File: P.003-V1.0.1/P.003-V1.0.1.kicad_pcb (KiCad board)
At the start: 2 copper layers, 19 parts, among them Q1 BS250, SW1 ON/OFF, SW2 Mode, SW3 Roll, U1 ATtiny85-20P, U2 74HC595

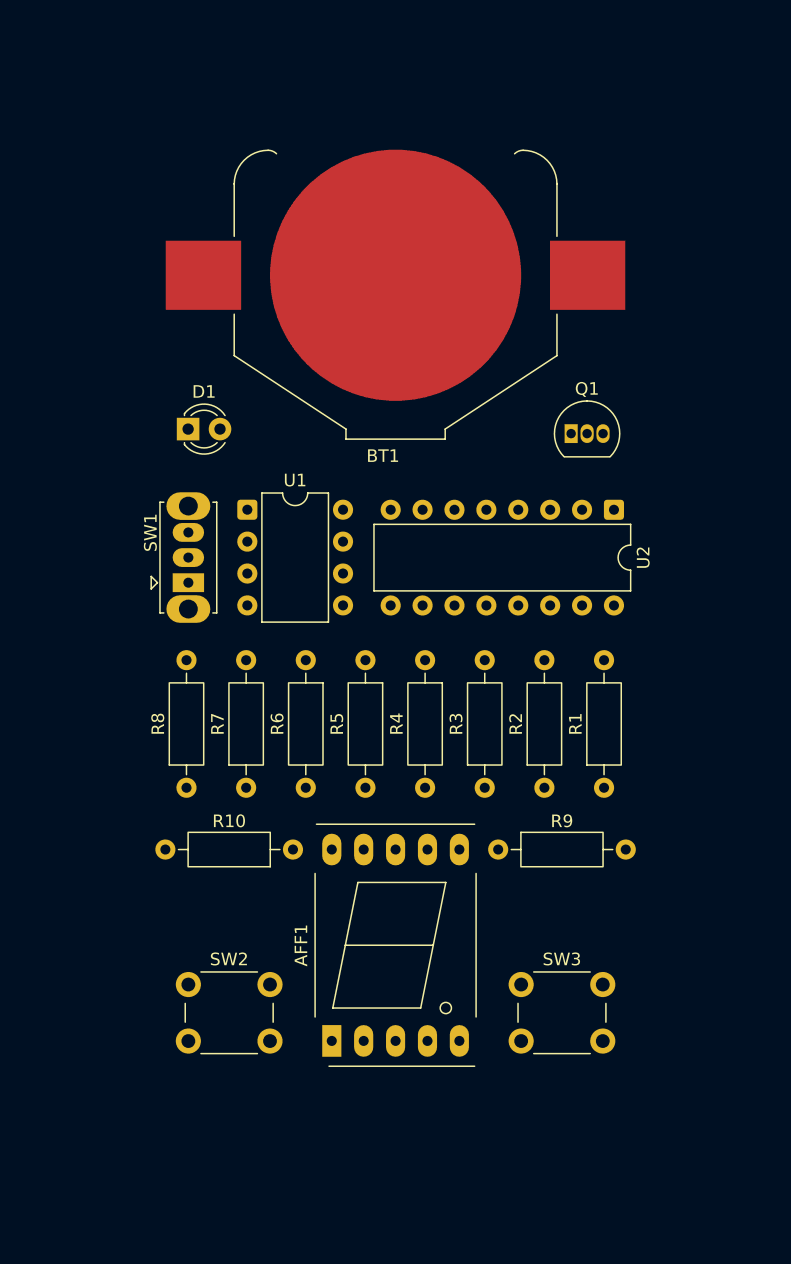
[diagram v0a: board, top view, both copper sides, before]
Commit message: add
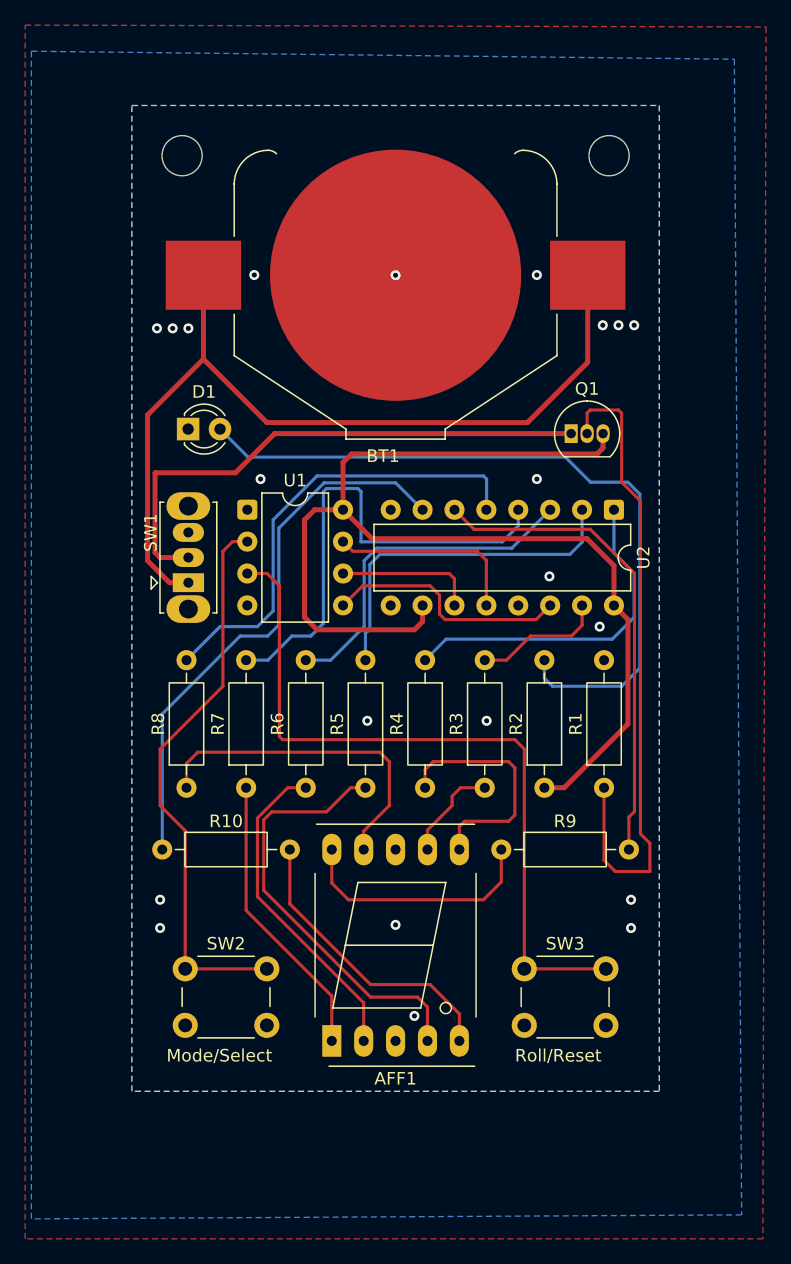
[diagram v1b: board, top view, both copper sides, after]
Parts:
- added ?: MountingHole_3.2mm_M3, MountingHole:MountingHole_3.2mm_M3, F.Cu at (112.0, 52.0)
- added ?: MountingHole_3.2mm_M3, MountingHole:MountingHole_3.2mm_M3, F.Cu at (146.0, 52.0)
- moved SW2 1.27 mm to (112.2, 116.7)
- moved SW3 1.27 mm to (139.2, 116.7)
- moved R10 0.25 mm to (120.6, 107.2)
- moved R9 0.25 mm to (137.4, 107.2)
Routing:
- net /Attiny85/VIN+: track 0.00 -> 93.8 mm
- net Net-(BT1-+): track 0.00 -> 70.2 mm
- net Net-(D1-A): track 0.00 -> 59.3 mm
- net Net-(U1-XTAL2/PB4): track 0.00 -> 58.9 mm
- net Net-(Q1-G): track 0.00 -> 51.8 mm
- net Net-(U1-XTAL1/PB3): track 0.00 -> 44.9 mm
- net /Display 7 Segment/Q7: track 0.00 -> 44.6 mm
- net Net-(Q1-D): track 0.00 -> 43.6 mm
- net /Display 7 Segment/Q4: track 0.00 -> 39.4 mm
- net /Display 7 Segment/Q6: track 0.00 -> 38.6 mm
- net /Display 7 Segment/Q5: track 0.00 -> 36.8 mm
- net Net-(AFF1-c): track 0.00 -> 34.4 mm
- net /Display 7 Segment/Q2: track 0.00 -> 28.0 mm
- net /Display 7 Segment/Q3: track 0.00 -> 27.5 mm
- net /Display 7 Segment/Q1: track 0.00 -> 27.3 mm
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- added copper zone on B.Cu, net /Attiny85/VIN-
- added copper zone on F.Cu, net /Attiny85/VIN-
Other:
- board outline added: 42 x 78.5 mm
- board text added: "GSAS - LABS P. 003 V. 1.0.1"
- board text added: "Mode/Select"
- board text added: "Roll/Reset"
